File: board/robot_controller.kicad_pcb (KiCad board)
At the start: 2 copper layers, 328 parts, among them J101 +3.3V, J102 +24V, J103 GND, J104 JTAG-ARM, J105 Power, J106 FTDI-USB, J107 Industrial Inputs, J108 Industrial Outputs, J109 MCU-USB, J110 AUX-USART6, J111 UEXT0, J112 UEXT1, J113 RGB LEDs, J201 Temp 0, J2301 Motor 0, J2302 Limit 0, J2401 Motor 1, J2402 Limit 1, J2501 Motor 2, J2502 Limit 2, J2601 Motor 3, J2602 Limit 3, J301 Temp 1, Q101 PNP, Q1501 NJT4031NT1G, Q1601 NJT4031NT1G, Q1701 NJT4031NT1G, Q1801 NJT4031NT1G, Q1901 NJT4031NT1G, Q2001 NJT4031NT1G, Q2101 NJT4031NT1G, Q2201 NJT4031NT1G, Q401 MMBT5962, Q402 MMBT5962, Q501 MMBT5962, Q502 MMBT5962, SW101 SW0, SW102 SW1, SW103 SW2, SW104 SW3, SW105 RESET, SW106 BOOT, U101 STM32F405-144, U102 FT232RL, U201 MAX6675, U2301 L6470, U2401 L6470, U2501 L6470, U2601 L6470, U301 MAX6675, U601 LMZ14201, X101 8MHZ

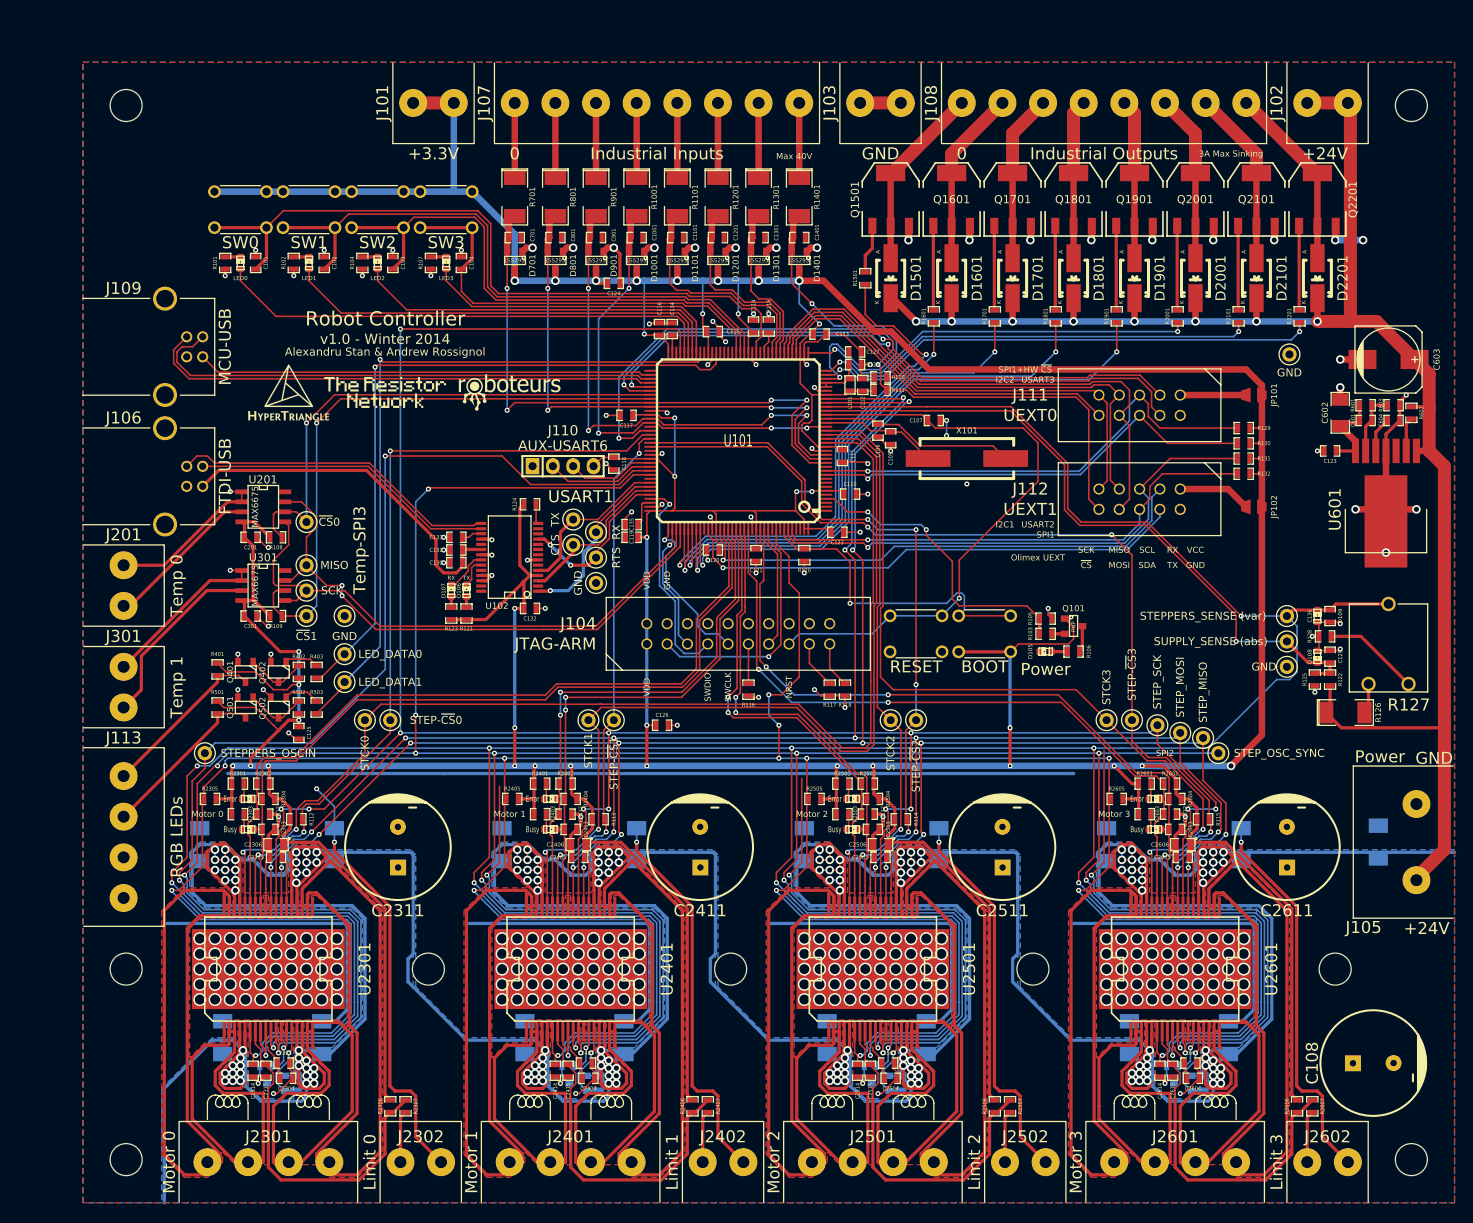
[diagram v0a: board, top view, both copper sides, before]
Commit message: Moved board in a cooler spot
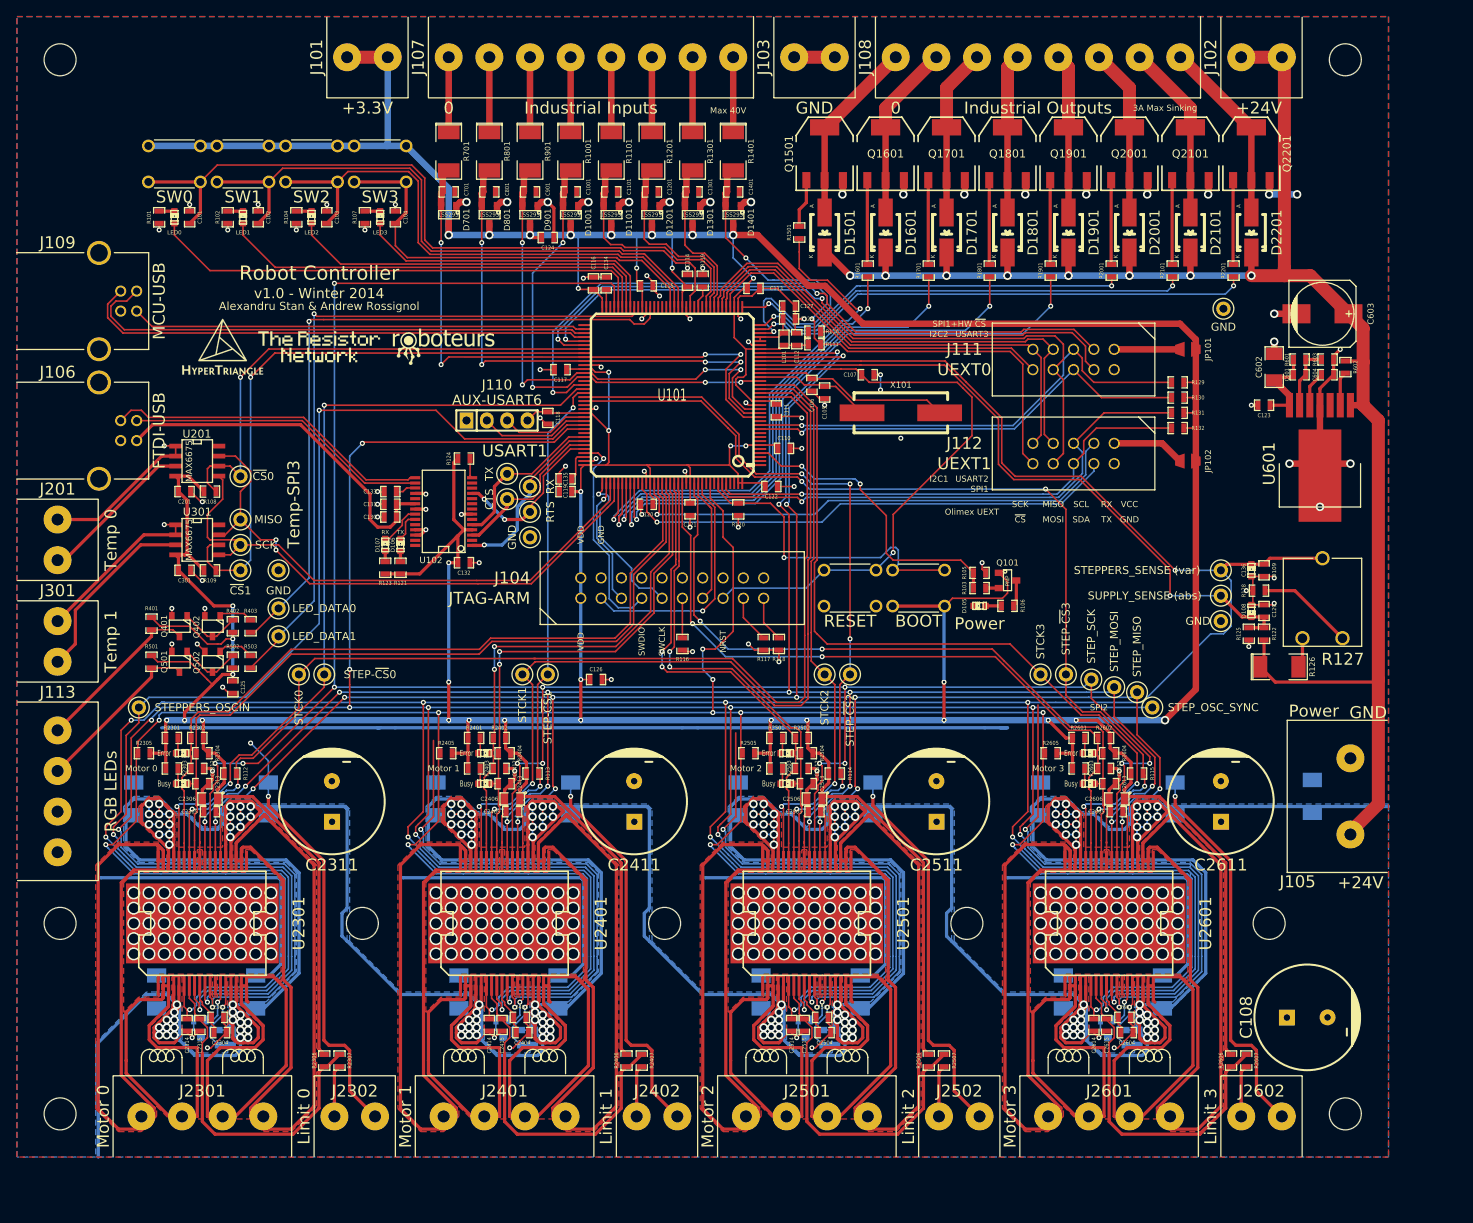
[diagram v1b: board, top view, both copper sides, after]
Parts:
- moved C2603 10.0 mm to (155.6, 142.9)
- moved C2611 10.0 mm to (167.6, 115.9)
- moved C2614 10.0 mm to (151.8, 143.8)
- moved C601 10.0 mm to (177.5, 62.5)
- moved D108 10.0 mm to (171.4, 92.1)
- moved D2201 10.0 mm to (171.4, 44.8)
- moved J2601 10.0 mm to (153.7, 155.3)
- moved JP101 10.0 mm to (163.5, 59.4)
- moved JP102 10.0 mm to (163.5, 73.3)
- moved MH 10.0 mm to (135.9, 131.1)
- moved Q2201 10.0 mm to (171.4, 34.9)
- moved R601 10.0 mm to (177.5, 60.6)
- moved SW106 10.0 mm to (129.9, 89.2)
- moved TP115 10.0 mm to (167.6, 93.3)
- moved TP128 10.0 mm to (167.6, 90.2)
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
